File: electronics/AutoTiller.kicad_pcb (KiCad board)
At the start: 4 copper layers, 135 x 32 mm, 92 parts, among them IC1 ESP32-C3-MINI-1-N4, J1 USB_C_Receptacle_USB2.0, J2 UART, SW1 Power, SW2 +1, SW3 -1, SW4 +15, SW5 -15, SW6 L, SW7 R, SW8 Reset

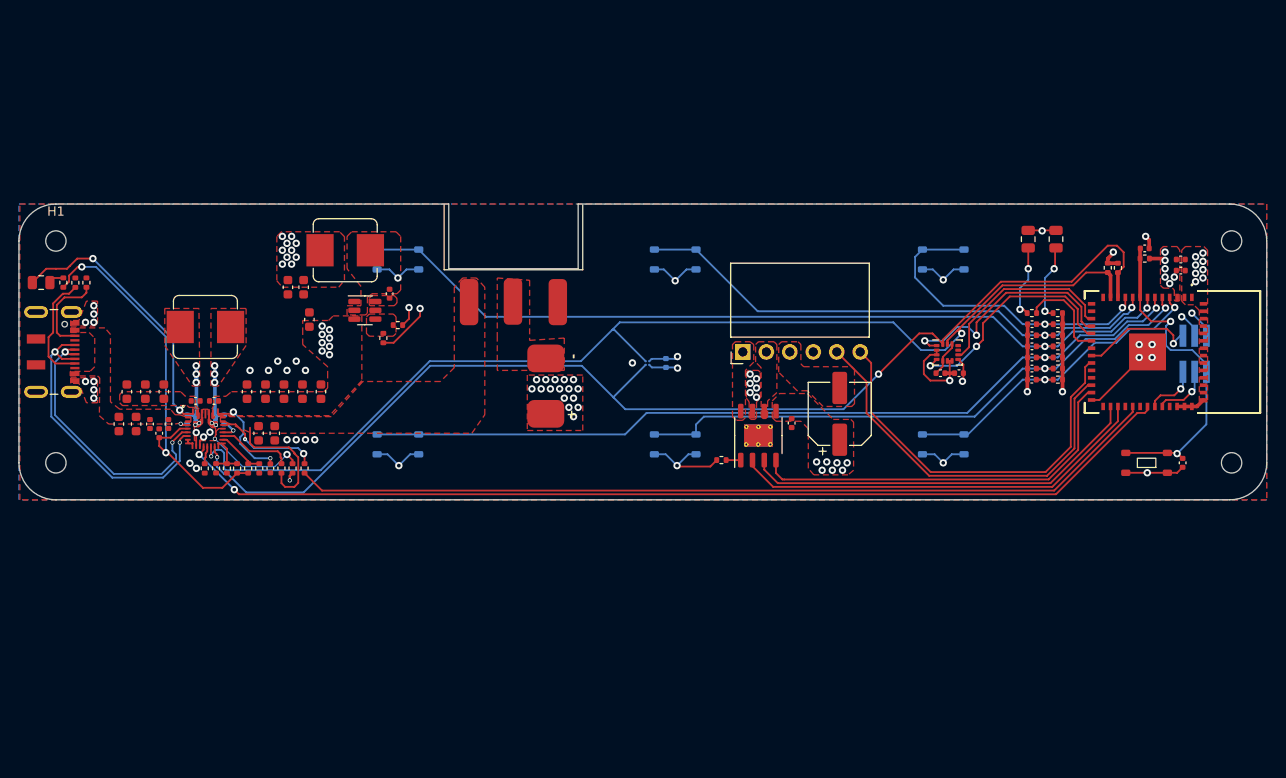
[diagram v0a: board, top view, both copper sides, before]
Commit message: Final Rev2 PCB
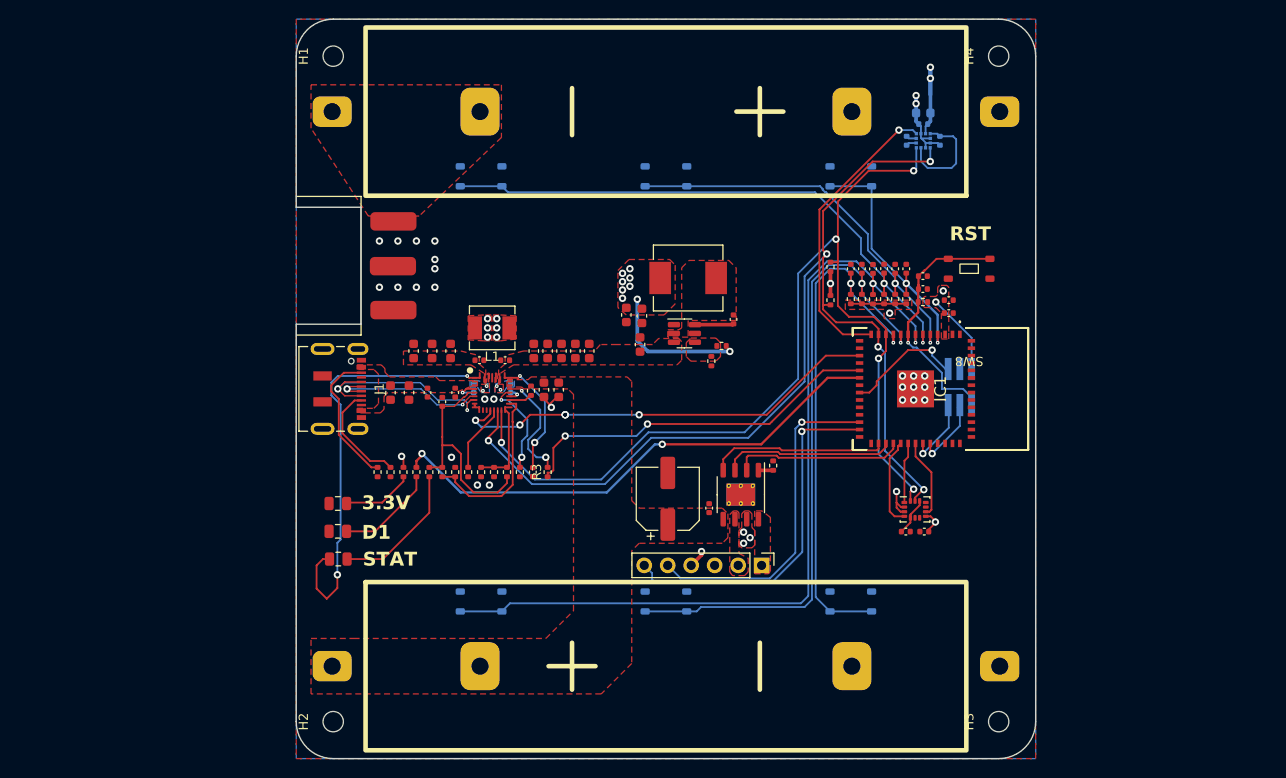
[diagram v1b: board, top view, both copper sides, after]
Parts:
- removed C43: 10u, Capacitor_SMD:C_0603_1608Metric
- removed L3: 1u, Inductor_SMD:L_Bourns_SRP7028A_7.3x6.6mm
- removed MMC5603NJ1: ~, Package_BGA:WLP-4_0.83x0.83mm_P0.4mm
- removed R27, R28: 10k, Resistor_SMD:R_0402_1005Metric
- added BT2: Battery, 18650:254 clip, F.Cu at (160.0, 90.0)
- added C1: 0.1u, Capacitor_SMD:C_0402_1005Metric, F.Cu at (134.2, 120.4)
- added C2: 0.1u, Capacitor_SMD:C_0402_1005Metric, F.Cu at (183.6, 107.0)
- added C3: 0.1u, Capacitor_SMD:C_0402_1005Metric, F.Cu at (137.2, 120.4)
- added C4: 10u, Capacitor_SMD:C_0603_1608Metric, F.Cu at (157.2, 115.2)
- added L1: 1u, Inductor_SMD:L_Sunlord_MWSA0402S, F.Cu at (141.2, 113.4)
- added R1: 47k, Resistor_SMD:R_0402_1005Metric, F.Cu at (183.6, 110.3)
- added R3: 10k, Resistor_SMD:R_0402_1005Metric, F.Cu at (147.2, 129.0)
- added U1: ~, Package_TO_SOT_SMD:TSOT-23-6, F.Cu at (162.0, 114.0)
- BT1: footprint XT30-U:XT30-U -> 18650:254 clip
- C11, C29: value 10u -> 0.1u; footprint Capacitor_SMD:C_0603_1608Metric -> Capacitor_SMD:C_0402_1005Metric
- C12: value 22u -> 0.1u; footprint Capacitor_SMD:C_0603_1608Metric -> Capacitor_SMD:C_0402_1005Metric
- C13: value 22u -> .1u; footprint Capacitor_SMD:C_0603_1608Metric -> Capacitor_SMD:C_0402_1005Metric
- C14: value 2.2uF -> 22u; footprint Capacitor_SMD:C_0402_1005Metric -> Capacitor_SMD:C_0603_1608Metric; moved to F.Cu
- C16, C19, C23, C24, C27, C5, C8: value 0.1u -> 10u; footprint Capacitor_SMD:C_0402_1005Metric -> Capacitor_SMD:C_0603_1608Metric
- C17: value 0.1u -> 4.7u
- C18: value 0.1u -> 22u; footprint Capacitor_SMD:C_0402_1005Metric -> Capacitor_SMD:C_0603_1608Metric
- C21: value 100n -> 0.1u
- C22: value 100n -> 10u; footprint Capacitor_SMD:C_0402_1005Metric -> Capacitor_SMD:C_0603_1608Metric
- C26: value 10u -> 22u; footprint Capacitor_SMD:C_0603_1608Metric -> Capacitor_SMD:C_0402_1005Metric
- C31: value 10u -> 1n; footprint Capacitor_SMD:C_0603_1608Metric -> Capacitor_SMD:C_0402_1005Metric
- C32: value 10u -> 1u; footprint Capacitor_SMD:C_0603_1608Metric -> Capacitor_SMD:C_0402_1005Metric
- C33: value 47n -> 10u; footprint Capacitor_SMD:C_0402_1005Metric -> Capacitor_SMD:C_0603_1608Metric; moved to F.Cu
- C34: value 47n -> 0.1u; moved to F.Cu
- C35, C42: value 10u -> 100n; footprint Capacitor_SMD:C_0603_1608Metric -> Capacitor_SMD:C_0402_1005Metric
- C36: value 10u -> 0.22u; footprint Capacitor_SMD:C_0603_1608Metric -> Capacitor_SMD:C_0402_1005Metric; moved to B.Cu
- C37: value 4.7u -> 0.1u; moved to B.Cu
- C39: value 1n -> 0.1u; moved to B.Cu
- C40: value .1u -> 47u; footprint Capacitor_SMD:C_0402_1005Metric -> Capacitor_SMD:CP_Elec_6.3x5.9
- C41: moved to B.Cu
- C6: value 47u -> 47n; footprint Capacitor_SMD:CP_Elec_6.3x5.9 -> Capacitor_SMD:C_0402_1005Metric; moved to B.Cu
- C7: value 22u -> 47n; moved to B.Cu
- C9: value 1u -> 0.1u
- L2: footprint Inductor_SMD:L_Bourns_SRP7028A_7.3x6.6mm -> Inductor_SMD:L_Sunlord_MWSA0618S
- R10: value 47k -> 100
- R11: value 47k -> 5.24k
- R12: value 47k -> 30.31k
- R13: value 47k -> 127k
- R14: value 47k -> 10k
- R15: value 127k -> 47k
- R16: value 100k -> 6.04k
- R17: value 5.24k -> 100k
- R18: value 30.31k -> 10k
- R19: value 10k -> 5.1k
- R2, R24, R25: value 5.1k -> 10k
- R22: value 100 -> 5.1k
- R23: value 10.5k -> 5.1k
- R4, R5, R6: value 10k -> 47k
- SW1: value Power -> +1; footprint Switch:0.5in_Slide -> Switch:Tactile_5.5mmx2.85mm; moved to B.Cu
- SW2: value +1 -> -1
- SW3: value -1 -> +15
- SW4: value +15 -> -15
- SW5: value -15 -> Power; footprint Switch:Tactile_5.5mmx2.85mm -> Switch:0.5in_Slide; moved to F.Cu
- U2: footprint Connector_PinHeader_2.54mm:PinHeader_1x06_P2.54mm_Horizontal -> Package_LGA:LGA-12_2x2mm_P0.5mm; moved to B.Cu
- U3: footprint Package_TO_SOT_SMD:TSOT-23-6 -> Connector_PinHeader_2.54mm:PinHeader_1x06_P2.54mm_Vertical
- moved C37 90.2 mm to (189.6, 93.2), turned to -90 degrees
- moved C26 88.9 mm to (190.6, 110.4), turned to 0 degrees
- moved C41 87.5 mm to (187.8, 90.2), turned to 180 degrees
- moved C8 84.7 mm to (132.2, 120.4), turned to -90 degrees
- moved C42 83.7 mm to (185.9, 135.4), turned to 0 degrees
- moved D1 82.8 mm to (124.5, 132.4), turned to 0 degrees
- moved D2 81.1 mm to (124.5, 135.4), turned to 0 degrees
- moved C39 79.9 mm to (187.8, 91.3), turned to 180 degrees
- moved R26 79.3 mm to (171.6, 128.3), turned to -90 degrees
- moved R18 78.6 mm to (187.8, 110.6), turned to 180 degrees
- moved C34 77.2 mm to (187.8, 107.8), turned to 0 degrees
- moved C36 76.9 mm to (186.0, 93.2), turned to 90 degrees
- moved C29 76.4 mm to (190.6, 111.8), turned to 0 degrees
- moved C7 73.6 mm to (143.2, 119.9), turned to -90 degrees
- moved R15 73.5 mm to (186.0, 110.3), turned to 90 degrees
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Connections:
- BT1 pad 1: Net-(BT1-+) -> VBAT
- BT1 pad 2: GND -> /BT1
- C10 pad 1: /BST -> +15
- C10 pad 2: /SW -> GND
- C11 pad 1: +12V -> /BST
- C11 pad 2: GND -> /SW
- C12 pad 1: +3.3V -> -15
- C13 pad 1: +3.3V -> /PMID
- C15 pad 1: +1 -> TackL
- C16 pad 1: -1 -> /PMID
- C17 pad 1: +15 -> REGN
- C18 pad 1: -15 -> +3.3V
- C19 pad 1: TackL -> /PMID
- C21 pad 1: +3.3V -> +12V
- C22 pad 1: Net-(LSM6DSMTR1-CS) -> /PMID
- C23 pad 1: VBUS -> +12V
- C24 pad 1: VBUS -> +12V
- C25 pad 1: VBUS -> VBAT
- C26 pad 1: VBUS -> +3.3V
- C28 pad 1: +12V -> VBAT
- C29 pad 1: +12V -> +3.3V
- C31 pad 1: +12V -> /SDRV
- C32 pad 1: +12V -> ESP_EN
- C33 pad 1: /BTST1 -> +12V
- C33 pad 2: /SW1 -> GND
- C34 pad 1: /SW2 -> ESP_EN
- C34 pad 2: /BTST2 -> GND
- C35 pad 1: VBAT -> +3.3V
- C36 pad 1: VBAT -> Net-(U2-C1)
- C37 pad 1: REGN -> Vdd_IO
- C38 pad 1: ESP_EN -> VBAT
- C39 pad 1: /SDRV -> +3.3V
- C40 pad 1: /PMID -> VBAT
- C41 pad 1: /PMID -> +3.3V
- C42 pad 1: /PMID -> Net-(LSM6DSMTR1-CS)
- C5 pad 1: +12V -> VBUS
- C6 pad 1: +12V -> /BTST1
- C6 pad 2: GND -> /SW1
- C7 pad 1: +3.3V -> /SW2
- C7 pad 2: GND -> /BTST2
- C8 pad 1: +3.3V -> VBUS
- C9 pad 1: ESP_EN -> -1
- DRV8251ADDAR1 pad 5: +12V -> VBAT
- IC1 pad 10: +1 -> TackL
- IC1 pad 13: unconnected-(IC1-IO25-Pad13) -> Compass_INT
- IC1 pad 16: IMU_INT2 -> QON
- IC1 pad 17: SAO -> unconnected-(IC1-IO12-Pad17)
- IC1 pad 18: IMU_INT1 -> BC_INT
- IC1 pad 22: ENC_B -> unconnected-(IC1-IO4-Pad22)
- IC1 pad 26: MC_VREF -> ENC_B
- IC1 pad 29: MC_IN1 -> MC_VREF
- IC1 pad 30: MC_IN2 -> MC_IN1
- IC1 pad 31: unconnected-(IC1-IO23-Pad31) -> MC_IN2
- IC1 pad 32: BC_INT -> IMU_INT1
- IC1 pad 33: unconnected-(IC1-IO22-Pad33) -> SAO
- IC1 pad 34: QON -> IMU_INT2
- IC1 pad 4: -1 -> TackR
- IC1 pad 5: -15 -> +15
- IC1 pad 6: TackL -> +1
- IC1 pad 7: TackR -> -1
- IC1 pad 9: +15 -> -15
- R10 pad 1: +3.3V -> /BATP
- R10 pad 2: -1 -> VBAT
- R11 pad 1: +3.3V -> REGN
- R11 pad 2: +15 -> /TS
- R12 pad 1: +3.3V -> /TS
- R12 pad 2: -15 -> GND
- R13 pad 1: +3.3V -> /ILIM_HIZ
- R13 pad 2: TackL -> REGN
- R14 pad 1: +3.3V -> /TS
- R14 pad 2: TackR -> GND
- R15 pad 1: /ILIM_HIZ -> +3.3V
- R15 pad 2: REGN -> TackR
- R16 pad 1: /ILIM_HIZ -> /PROG
- R17 pad 1: REGN -> /ILIM_HIZ
- R17 pad 2: /TS -> GND
- R18 pad 1: /TS -> +3.3V
- R18 pad 2: GND -> ESP_EN
- R19 pad 1: /TS -> +3.3V
- R19 pad 2: GND -> Net-(D1-A)
- R2 pad 2: Net-(DRV8251ADDAR1-IPROPI) -> /CE
- R20 pad 1: Net-(J1-CC2) -> S_LED
- R20 pad 2: GND -> Net-(D2-A)
- R21 pad 1: Net-(J1-CC1) -> REGN
- R21 pad 2: GND -> Net-(D3-A)
- R22 pad 1: /BATP -> Net-(J1-CC2)
- R22 pad 2: VBAT -> GND
- R23 pad 1: /PROG -> Net-(J1-CC1)
- R24 pad 2: Net-(D1-A) -> SCL
- R25 pad 1: S_LED -> +3.3V
- R25 pad 2: Net-(D2-A) -> SDA
- R26 pad 1: REGN -> GND
- R26 pad 2: Net-(D3-A) -> Net-(DRV8251ADDAR1-IPROPI)
- R4 pad 2: ESP_EN -> -1
- R5 pad 2: SDA -> +15
- R6 pad 2: SCL -> -15
- R9 pad 2: +1 -> TackL
- SW1 pad 1: VBAT -> GND
- SW1 pad 2: Net-(BT1-+) -> +1
- SW2 pad 2: +1 -> -1
- SW3 pad 2: -1 -> +15
- SW4 pad 2: +15 -> -15
- SW5 pad 1: GND -> unconnected-(SW5A-A-Pad1)
- SW5 pad 2: -15 -> GND
- U2 pad 1: /OUT1 -> SCL
- U2 pad 2: /OUT2 -> GND
- U2 pad 3: GND -> Vdd_IO
- U2 pad 4: +3.3V -> SDA
- U2 pad 5: ENC_A -> Net-(U2-C1)
- U2 pad 6: ENC_B -> GND
- U3 pad 1: GND -> /OUT1
- U3 pad 2: /SW -> /OUT2
- U3 pad 3: +12V -> GND
- U3 pad 4: /FB -> +3.3V
- U3 pad 5: 5V_EN -> ENC_A
- U3 pad 6: /BST -> ENC_B
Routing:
- net GND: track 92.7 -> 16.8 mm, vias 73 -> 31
- net TackR: track 92.3 -> 27.6 mm
- net QON: track 109.6 -> 47.5 mm, vias 2 -> 5
- net -1: track 36.2 -> 93.2 mm
- net BC_INT: track 94.5 -> 40.4 mm, vias 0 -> 2
- net S_LED: track 10.4 -> 56.2 mm, vias 0 -> 2
- net TackL: track 93.0 -> 57.8 mm
- net Compass_INT: track 0.00 -> 31.8 mm, vias 0 -> 1
- net MC_IN2: track 45.7 -> 18.4 mm
- net +1: track 36.2 -> 63.0 mm
- net MC_IN1: track 43.6 -> 18.6 mm
- net +3.3V: track 24.2 -> 48.8 mm, vias 22 -> 18
- net MC_VREF: track 42.7 -> 19.2 mm
- net REGN: track 44.6 -> 24.2 mm, vias 2 -> 0
- net SAO: track 25.7 -> 6.56 mm, vias 2 -> 0
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- added copper zone on In1.Cu, net /BT1
- added copper zone on B.Cu, net /SW1
- added copper zone on In1.Cu, net /SW1
- added copper zone on In2.Cu, net /SW1
- added copper zone on B.Cu, net /SW2
- added copper zone on In1.Cu, net /SW2
- added copper zone on In2.Cu, net /SW2
- added copper zone on F.Cu, net BT2
- removed copper zone on In1.Cu, net +12V
- removed copper zone on F.Cu, net /BST
- removed copper zone on F.Cu, net Net-(BT1-+)
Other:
- board size 135 x 32 mm -> 80 x 80 mm
- board text added: "3.3V"
- board text added: "D1"
- board text added: "RST"
- board text added: "STAT"
- board text removed: "+1"
- board text removed: "-1"
- board text removed: "-15"
- board text removed: "<Tack"
- board text removed: "OFF"
- board text removed: "ON"
- board text removed: "Tack>"
